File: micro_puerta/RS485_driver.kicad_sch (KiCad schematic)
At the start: 0 parts

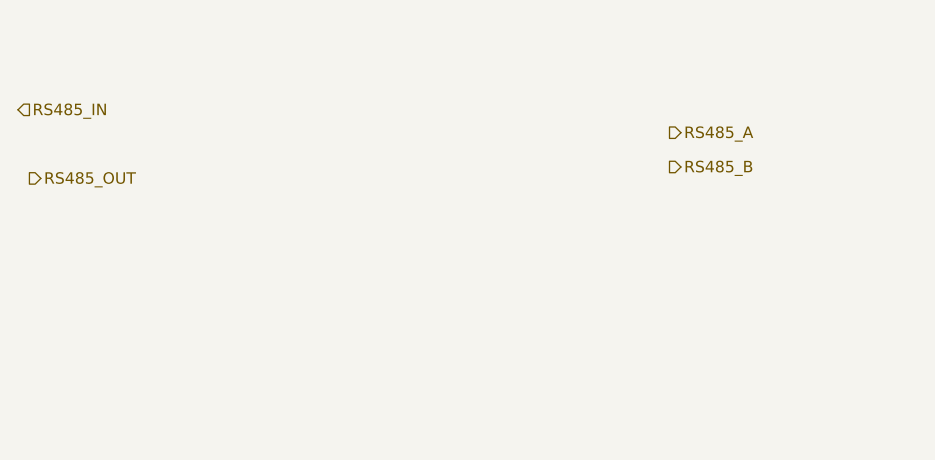
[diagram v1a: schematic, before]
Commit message: Actualizacion
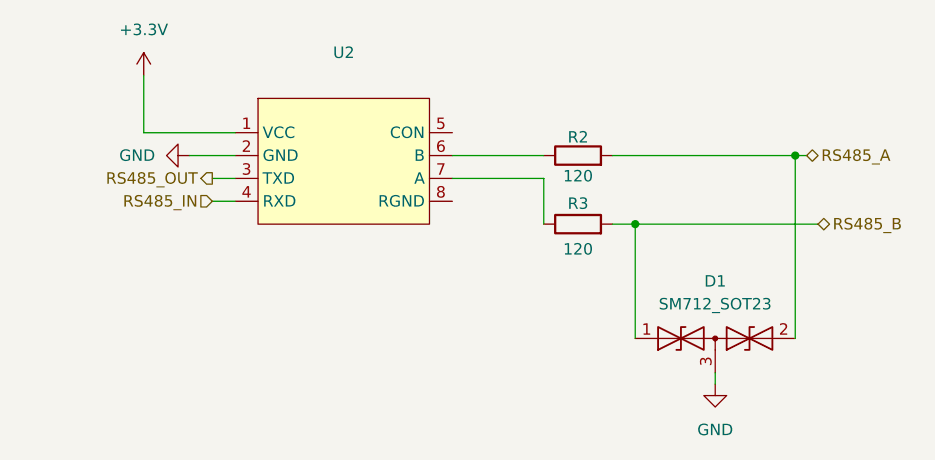
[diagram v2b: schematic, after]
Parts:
- added D1: SM712_SOT23, Package_TO_SOT_SMD:SOT-23, symbol Diode:SM712_SOT23
- added R2, R3: 120, symbol Device:R
- added U2: ~, Proyecto_componente:RSM3485ECHT, symbol Proyecto_componente:RSM3485ECHT
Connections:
- net RS485_A: now also D1.2 (A2), R2.2
- net RS485_B: now also D1.1 (A1), R3.2
- net RS485_IN: now also U2.4 (RXD)
- net RS485_OUT: now also U2.3 (TXD)
- new net: R2.1, U2.6 (B)
- new net: R3.1, U2.7 (A)
- new net +3.3V: U2.1 (VCC)
- new net GND: D1.3 (common), U2.2 (GND)
